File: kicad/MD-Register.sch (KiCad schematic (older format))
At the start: 0 parts

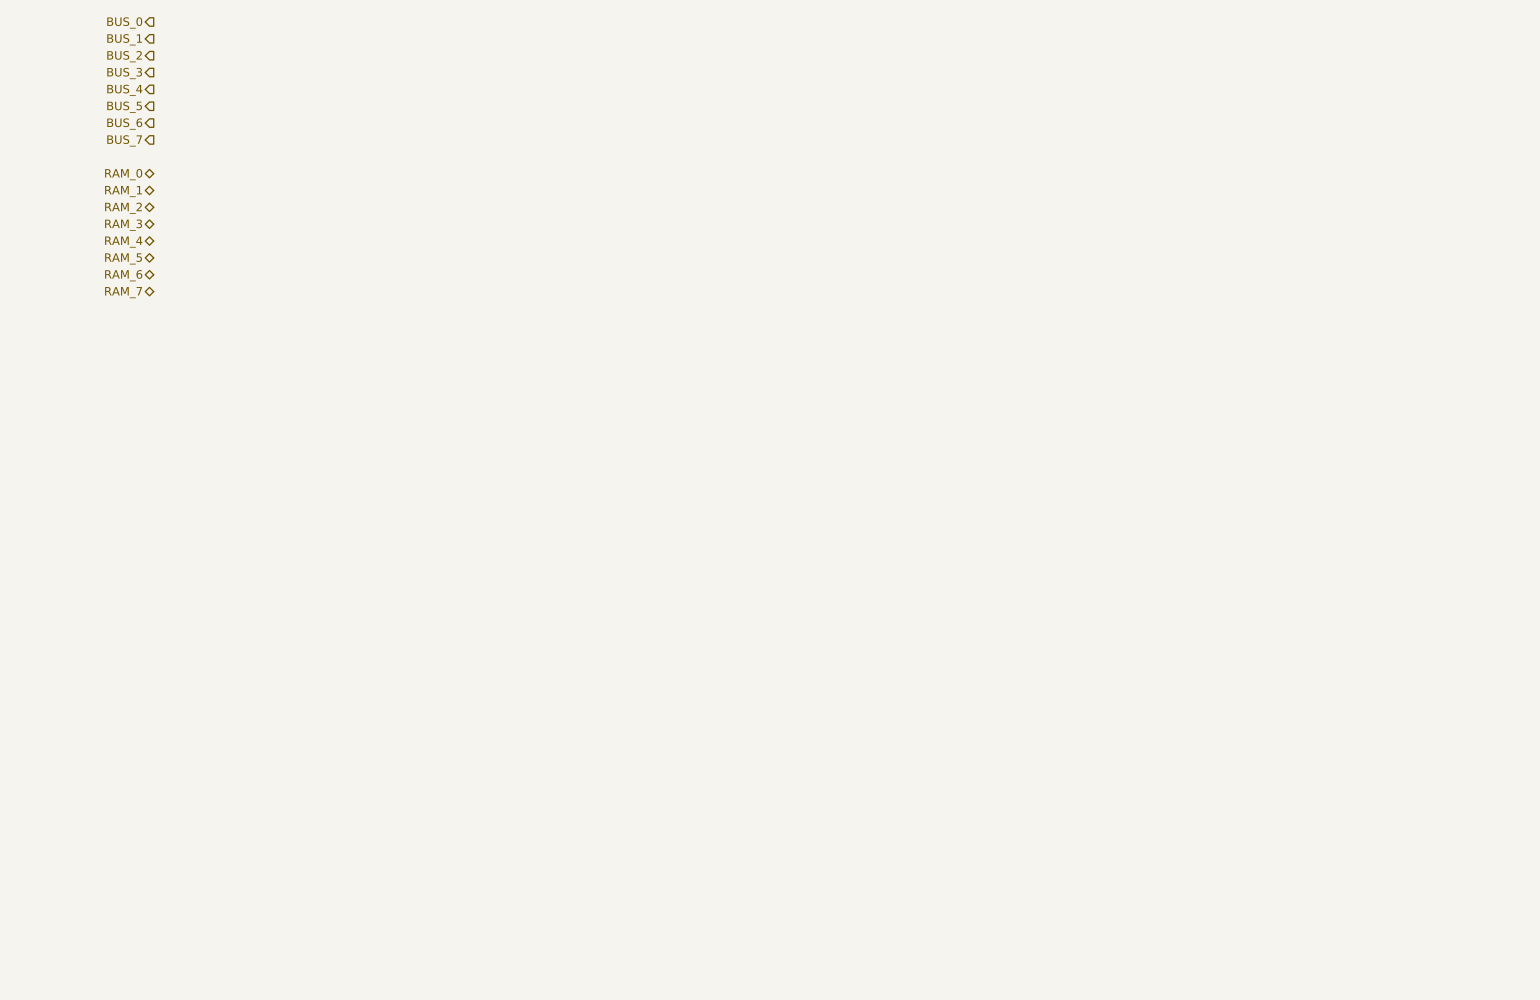
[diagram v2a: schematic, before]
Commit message: Finish todo list
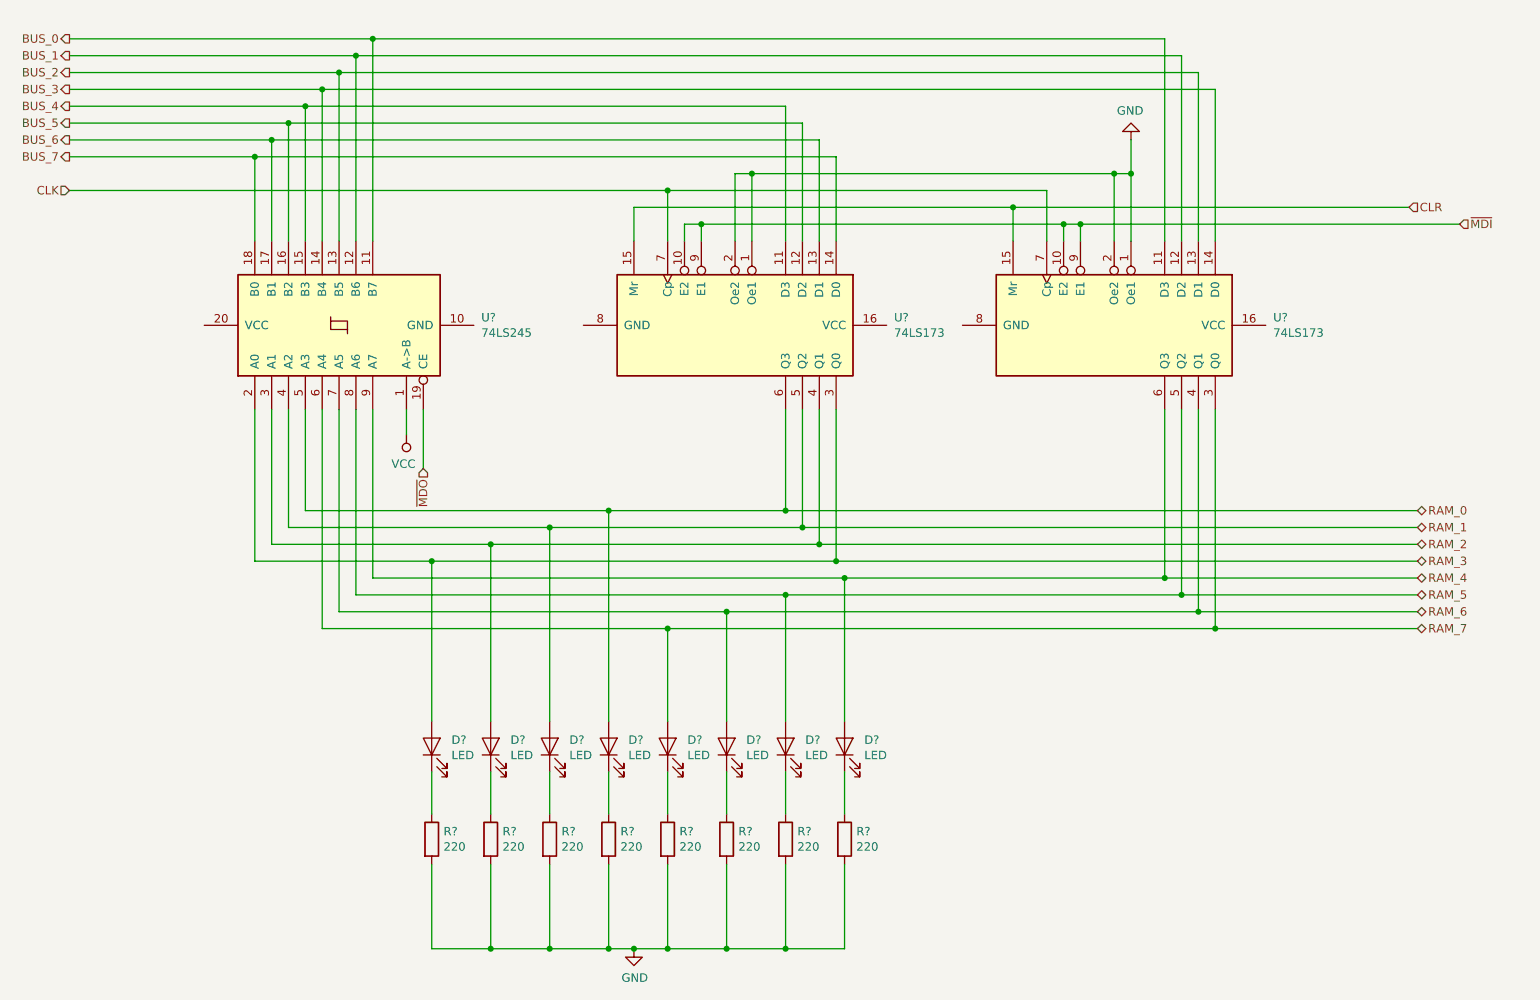
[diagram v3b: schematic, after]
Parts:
- added D? (x8): LED, symbol Device:LED
- added R? (x8): 220, symbol Device:R
- added U?: 74LS245, symbol 74xx:74LS245
- added U? (x2): 74LS173, symbol 74xx:74LS173
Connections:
- net BUS_0: now also U?.11 (B7), U?.11 (D3)
- net BUS_1: now also U?.12 (B6), U?.12 (D2)
- net BUS_2: now also U?.13 (B5), U?.13 (D1)
- net BUS_3: now also U?.14 (B4), U?.14 (D0)
- net BUS_4: now also U?.11 (D3), U?.15 (B3)
- net BUS_5: now also U?.12 (D2), U?.16 (B2)
- net BUS_6: now also U?.13 (D1), U?.17 (B1)
- net BUS_7: now also U?.14 (D0), U?.18 (B0)
- net RAM_0: now also D?.2 (A), U?.5 (A3), U?.6 (Q3)
- net RAM_1: now also D?.2 (A), U?.4 (A2), U?.5 (Q2)
- net RAM_2: now also D?.2 (A), U?.3 (A1), U?.4 (Q1)
- net RAM_3: now also D?.2 (A), U?.2 (A0), U?.3 (Q0)
- net RAM_4: now also D?.2 (A), U?.6 (Q3), U?.9 (A7)
- net RAM_5: now also D?.2 (A), U?.5 (Q2), U?.8 (A6)
- net RAM_6: now also D?.2 (A), U?.4 (Q1), U?.7 (A5)
- net RAM_7: now also D?.2 (A), U?.3 (Q0), U?.6 (A4)
- new net: D?.1 (K), R?.1 (x8)
- new net CLK: U?.7 (Cp), U?.7 (Cp)
- new net CLR: U?.15 (Mr), U?.15 (Mr)
- new net GND: R?.2, R?.2, R?.2, R?.2, R?.2, R?.2, R?.2, R?.2, U?.1 (Oe1), U?.1 (Oe1), U?.2 (Oe2), U?.2 (Oe2)
- new net VCC: U?.1 (A->B)
- new net ~MDI~: U?.10 (E2), U?.10 (E2), U?.9 (E1), U?.9 (E1)
- new net ~MDO~: U?.19 (CE)
